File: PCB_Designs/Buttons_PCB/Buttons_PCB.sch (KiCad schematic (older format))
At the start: 71 parts, among them P1 CONN_01X05, P2 CONN_01X01, P3 CONN_01X01, P4 CONN_01X01, U1 CHERRY-MX, U10 CHERRY-MX, U11 CHERRY-MX, U12 CHERRY-MX, U13 MCP23017, U14 MCP23017, U2 CHERRY-MX, U3 CHERRY-MX, U4 CHERRY-MX, U5 CHERRY-MX, U6 CHERRY-MX, U7 CHERRY-MX, U8 CHERRY-MX, U9 CHERRY-MX

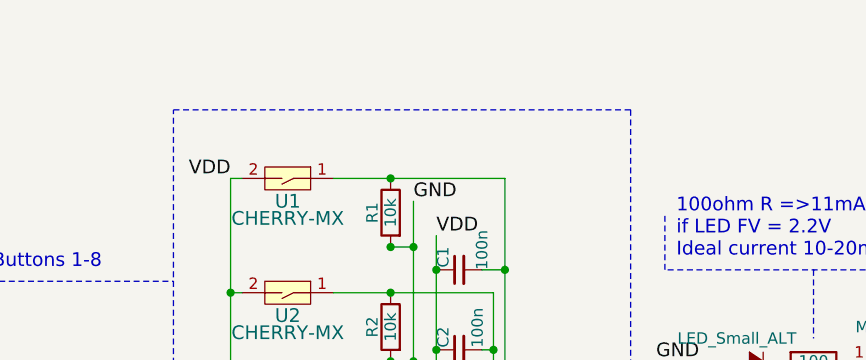
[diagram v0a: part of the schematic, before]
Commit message: First PCB version of main board
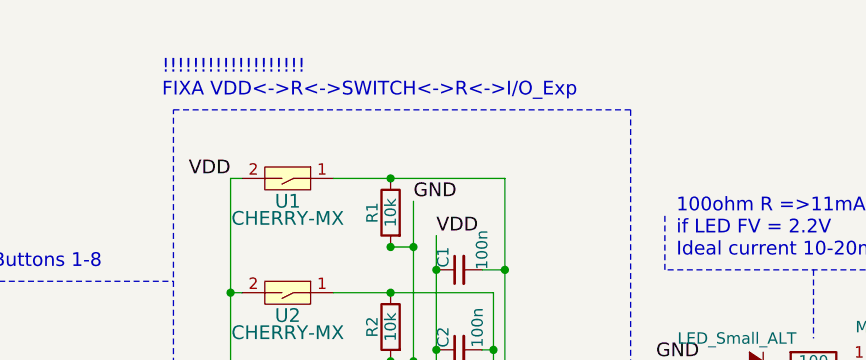
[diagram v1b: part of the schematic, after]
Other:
- note added: "!!!!!!!!!!!!!!!!!!!"
- note added: "FIXA VDD<->R<->SWITCH<->R<->I/O_Exp"
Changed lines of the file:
@@
 VDD
 $Comp
-L PWR_FLAG #FLG1
+L PWR_FLAG #FLG01
 U 1 1 588ED4C3
 P 7150 750
-F 0 "#FLG1" H 7150 825 50  0001 C CNN
+F 0 "#FLG01" H 7150 825 50  0001 C CNN
 F 1 "PWR_FLAG" H 7150 900 50  0000 C CNN
 F 2 "" H 7150 750 50  0001 C CNN
@@
 $EndComp
 $Comp
-L PWR_FLAG #FLG2
+L PWR_FLAG #FLG02
 U 1 1 588ED59B
 P 7200 850
-F 0 "#FLG2" H 7200 925 50  0001 C CNN
+F 0 "#FLG02" H 7200 925 50  0001 C CNN
 F 1 "PWR_FLAG" H 7200 1000 50  0000 C CNN
 F 2 "" H 7200 850 50  0001 C CNN
@@
 Wire Wire Line
 	9000 2100 9000 2000
+Text Notes 3300 900  0    60   ~ 0
+FIXA VDD<->R<->SWITCH<->R<->I/O_Exp
+Text Notes 3300 800  0    60   ~ 0
+!!!!!!!!!!!!!!!!!!!
 $EndSCHEMATC
